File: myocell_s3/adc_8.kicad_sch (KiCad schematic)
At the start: 79 parts, among them U2 ADS1298xPAG

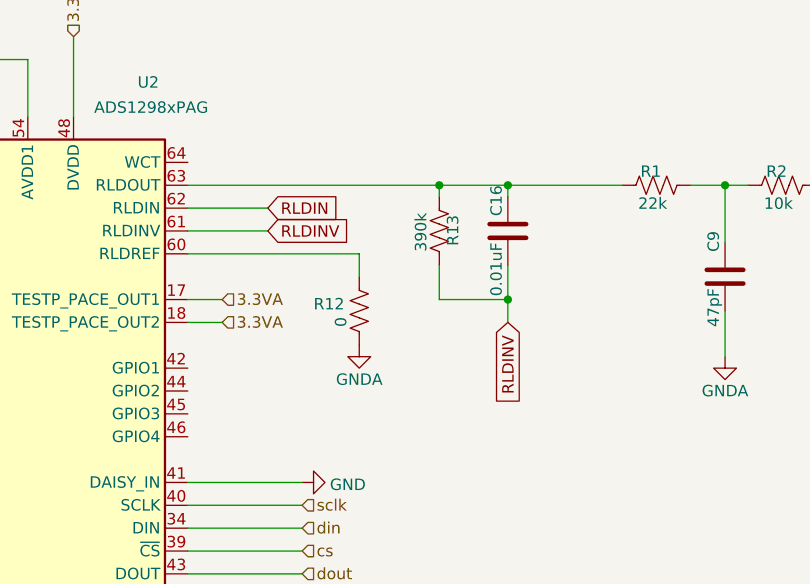
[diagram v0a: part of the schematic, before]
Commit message: schematic and footprints done
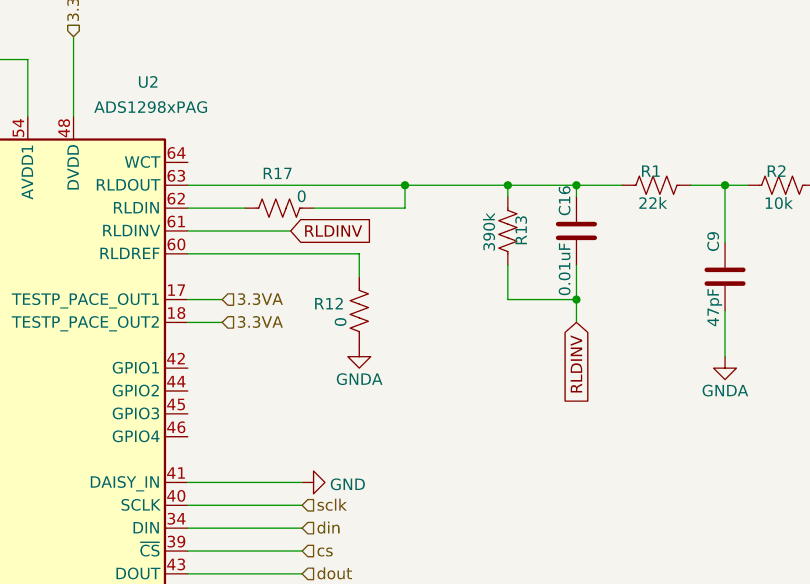
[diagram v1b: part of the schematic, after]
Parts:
- added R17: 0, Resistor_SMD:R_0805_2012Metric_Pad1.20x1.40mm_HandSolder, symbol Device:R_US
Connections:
- net at C16.2, R1.1, R13.1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: now also R17.1
- net RLDIN: no longer names the net of U2.62 (RLDIN)
- net RLDIN: now also R17.2
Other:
- moved on the sheet: C16, R13
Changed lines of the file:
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@@
 	)
 	(junction
-		(at 205.74 53.34)
+		(at 213.36 53.34)
 		(diameter 0)
 		(color 0 0 0 0)
@@
 	)
 	(junction
-		(at 213.36 53.34)
+		(at 220.98 53.34)
 		(diameter 0)
 		(color 0 0 0 0)
 	)
 	(junction
-		(at 213.36 66.04)
+		(at 201.93 53.34)
+		(diameter 0)
+		(color 0 0 0 0)
+	)
+	(junction
+		(at 220.98 66.04)
 		(diameter 0)
 		(color 0 0 0 0)
@@
 	(wire
 		(pts
-			(xy 205.74 66.04) (xy 205.74 62.23)
+			(xy 213.36 66.04) (xy 213.36 62.23)
 		)
 		(stroke
@@
 	(wire
 		(pts
-			(xy 213.36 66.04) (xy 213.36 68.58)
+			(xy 220.98 66.04) (xy 220.98 68.58)
 		)
 		(stroke
@@
 	(wire
 		(pts
-			(xy 213.36 53.34) (xy 226.06 53.34)
+			(xy 220.98 53.34) (xy 226.06 53.34)
 		)
 		(stroke
@@
 	(wire
 		(pts
-			(xy 213.36 62.23) (xy 213.36 66.04)
+			(xy 220.98 62.23) (xy 220.98 66.04)
 		)
 		(stroke
@@
 	(wire
 		(pts
-			(xy 177.8 55.88) (xy 186.69 55.88)
+			(xy 177.8 55.88) (xy 184.15 55.88)
 		)
 		(stroke
@@
 	(wire
 		(pts
+			(xy 201.93 53.34) (xy 213.36 53.34)
+		)
+		(stroke
+			(width 0)
+			(type default)
+		)
+	)
+	(wire
+		(pts
 			(xy 31.75 138.43) (xy 31.75 137.16)
 		)
@@
 	(wire
 		(pts
-			(xy 177.8 53.34) (xy 205.74 53.34)
+			(xy 177.8 53.34) (xy 201.93 53.34)
 		)
 		(stroke
@@
 	(wire
 		(pts
-			(xy 205.74 53.34) (xy 213.36 53.34)
+			(xy 213.36 53.34) (xy 220.98 53.34)
 		)
 		(stroke
@@
 	(wire
 		(pts
-			(xy 177.8 58.42) (xy 186.69 58.42)
+			(xy 177.8 58.42) (xy 189.23 58.42)
 		)
 		(stroke
@@
 	(wire
 		(pts
+			(xy 201.93 55.88) (xy 201.93 53.34)
+		)
+		(stroke
+			(width 0)
+			(type default)
+		)
+	)
+	(wire
+		(pts
 			(xy 59.69 83.82) (xy 59.69 85.09)
 		)
@@
 	(wire
 		(pts
-			(xy 205.74 53.34) (xy 205.74 54.61)
+			(xy 213.36 53.34) (xy 213.36 54.61)
 		)
 		(stroke
@@
 	(wire
 		(pts
-			(xy 213.36 53.34) (xy 213.36 54.61)
+			(xy 220.98 53.34) (xy 220.98 54.61)
 		)
 		(stroke
@@
 	(wire
 		(pts
+			(xy 191.77 55.88) (xy 201.93 55.88)
+		)
+		(stroke
+			(width 0)
+			(type default)
+		)
+	)
+	(wire
+		(pts
 			(xy 270.51 121.92) (xy 264.16 121.92)
 		)
@@
 	(wire
 		(pts
-			(xy 213.36 66.04) (xy 205.74 66.04)
+			(xy 220.98 66.04) (xy 213.36 66.04)
 		)
 		(stroke
@@
 	(global_label "RLDINV"
 		(shape input)
-		(at 213.36 68.58 270)
+		(at 220.98 68.58 270)
 		(fields_autoplaced yes)
 		(effects
@@
 		)
 		(property "Intersheetrefs" "${INTERSHEET_REFS}"
-			(at 213.36 78.1572 90)
+			(at 220.98 78.1572 90)
 			(effects
 				(font
@@
 	(global_label "RLDINV"
 		(shape input)
-		(at 186.69 58.42 0)
-		(fields_autoplaced yes)
-		(effects
-			(font
-				(size 1.27 1.27)
-			)
-			(justify left)
-		)
-		(property "Intersheetrefs" "${INTERSHEET_REFS}"
-			(at 196.2672 58.42 0)
-			(effects
-				(font
-					(size 1.27 1.27)
-				)
-				(justify left)
-				(hide yes)
-			)
-		)
-	)
-	(global_label "RLDIN"
-		(shape input)
-		(at 186.69 55.88 0)
+		(at 189.23 58.42 0)
 		(fields_autoplaced yes)
 		(effects
@@
 		)
 		(property "Intersheetrefs" "${INTERSHEET_REFS}"
-			(at 195.1786 55.88 0)
+			(at 198.8072 58.42 0)
 			(effects
 				(font
@@
 	(symbol
 		(lib_id "Device:C")
-		(at 213.36 58.42 180)
+		(at 220.98 58.42 180)
 		(unit 1)
 		(exclude_from_sim no)
@@
 		(dnp no)
 		(property "Reference" "C16"
-			(at 212.09 53.34 90)
+			(at 219.71 53.34 90)
 			(effects
 				(font
@@
 		)
 		(property "Value" "0.01uF"
-			(at 212.09 59.69 90)
+			(at 219.71 59.69 90)
 			(effects
 				(font
@@
 		)
 		(property "Footprint" "Capacitor_SMD:C_0805_2012Metric_Pad1.18x1.45mm_HandSolder"
-			(at 212.3948 54.61 0)
+			(at 220.0148 54.61 0)
 			(effects
 				(font
@@
 		)
 		(property "Datasheet" "~"
-			(at 213.36 58.42 0)
+			(at 220.98 58.42 0)
 			(effects
 				(font
@@
 		)
 		(property "Description" "Unpolarized capacitor"
-			(at 213.36 58.42 0)
+			(at 220.98 58.42 0)
 			(effects
 				(font
@@
 	(symbol
 		(lib_id "Device:R_US")
-		(at 205.74 58.42 0)
+		(at 213.36 58.42 0)
 		(unit 1)
 		(exclude_from_sim no)
@@
 		(dnp no)
 		(property "Reference" "R13"
-			(at 207.264 56.642 90)
+			(at 214.884 56.642 90)
 			(effects
 				(font
@@
 		)
 		(property "Value" "390k"
-			(at 203.708 56.388 90)
+			(at 211.328 56.388 90)
 			(effects
 				(font
@@
 		)
 		(property "Footprint" "Resistor_SMD:R_0805_2012Metric_Pad1.20x1.40mm_HandSolder"
-			(at 206.756 58.674 90)
+			(at 214.376 58.674 90)
 			(effects
 				(font
@@
 		)
 		(property "Datasheet" "~"
-			(at 205.74 58.42 0)
+			(at 213.36 58.42 0)
 			(effects
 				(font
@@
 		)
 		(property "Description" "Resistor, US symbol"
-			(at 205.74 58.42 0)
+			(at 213.36 58.42 0)
 			(effects
 				(font
@@
 					(unit 1)
 				)
+			)
+		)
+	)
+	(symbol
+		(lib_id "Device:R_US")
+		(at 187.96 55.88 270)
+		(unit 1)
+		(exclude_from_sim no)
+		(in_bom yes)
+		(on_board yes)
+		(dnp no)
+		(property "Reference" "R17"
+			(at 189.484 52.07 90)
+			(effects
+				(font
+					(size 1.27 1.27)
+				)
+				(justify right)
+			)
+		)
+		(property "Value" "0"
+			(at 191.008 54.61 90)
+			(effects
+				(font
+					(size 1.27 1.27)
+				)
+				(justify right)
+			)
+		)
+		(property "Footprint" "Resistor_SMD:R_0805_2012Metric_Pad1.20x1.40mm_HandSolder"
+			(at 187.706 56.896 90)
+			(effects
+				(font
+					(size 1.27 1.27)
+				)
+				(hide yes)
+			)
+		)
+		(property "Datasheet" "~"
+			(at 187.96 55.88 0)
+			(effects
+				(font
+					(size 1.27 1.27)
+				)
+				(hide yes)
+			)
+		)
+		(property "Description" "Resistor, US symbol"
+			(at 187.96 55.88 0)
+			(effects
+				(font
+					(size 1.27 1.27)
+				)
+				(hide yes)
+			)
+		)
+		(pin "1"
+		)
+		(pin "2"
+		)
+		(instances
+			(project "myocell_s3"
+				(path "/871ff10b-bde5-471c-b91a-de58aa271388/c595076a-24ce-4f55-8e02-687765014fdd"
+					(reference "R17")
+					(unit 1)
+				)

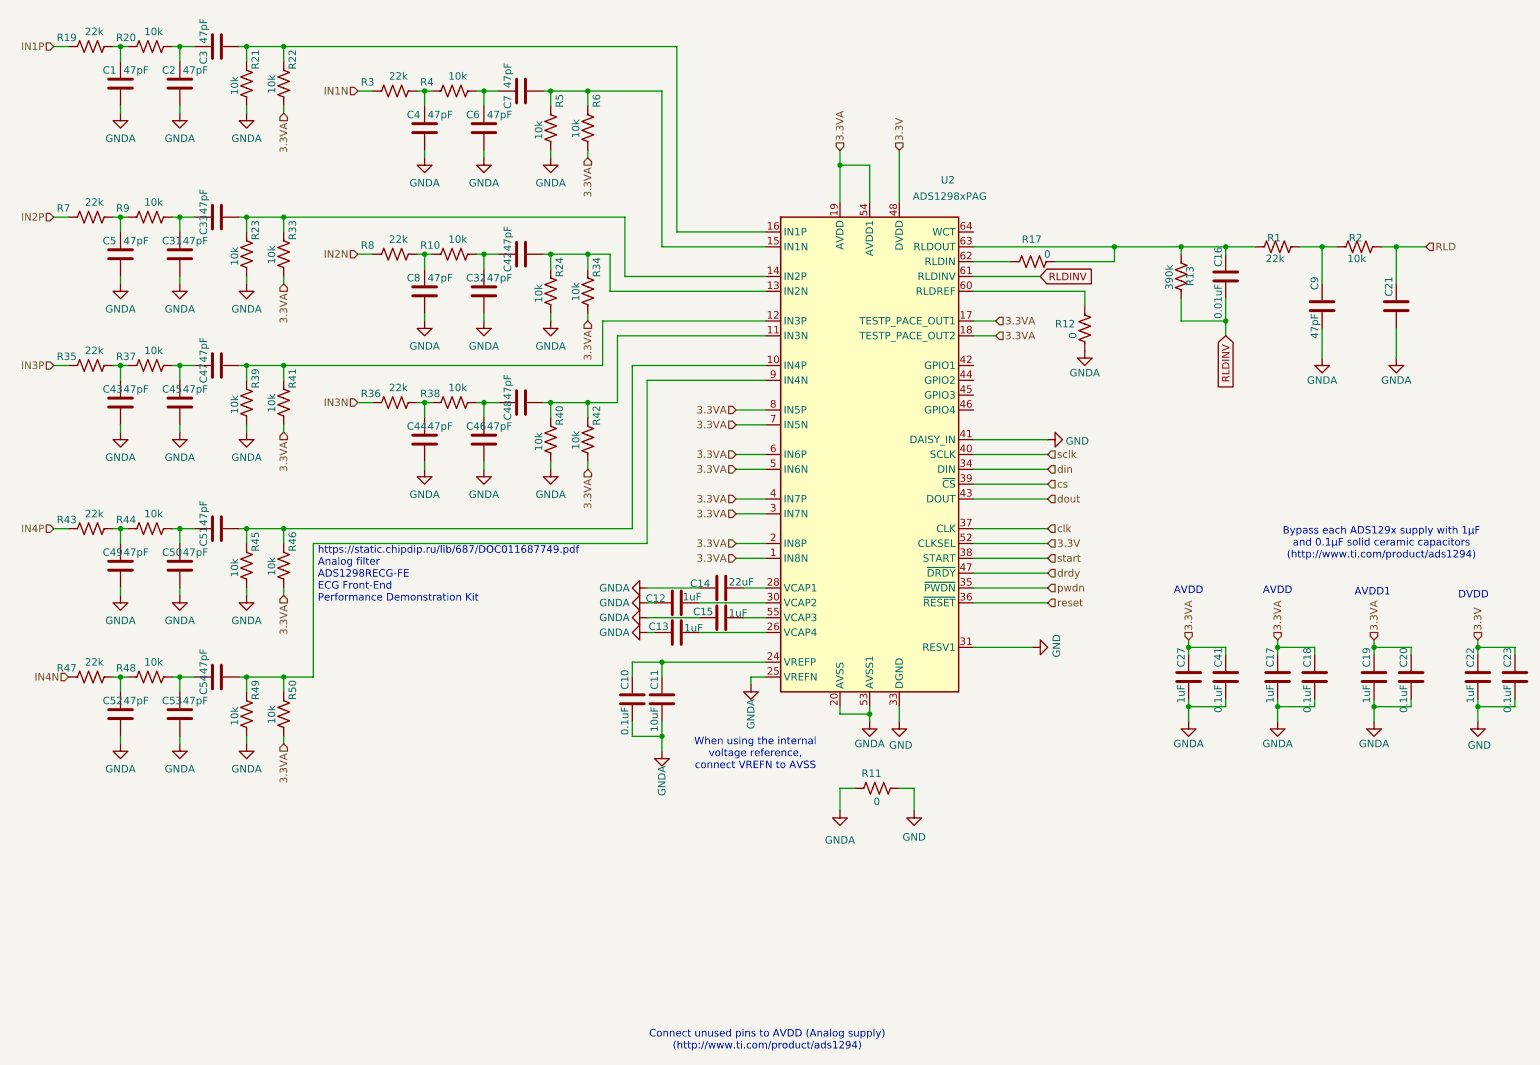
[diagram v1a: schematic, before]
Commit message: working on parts placement
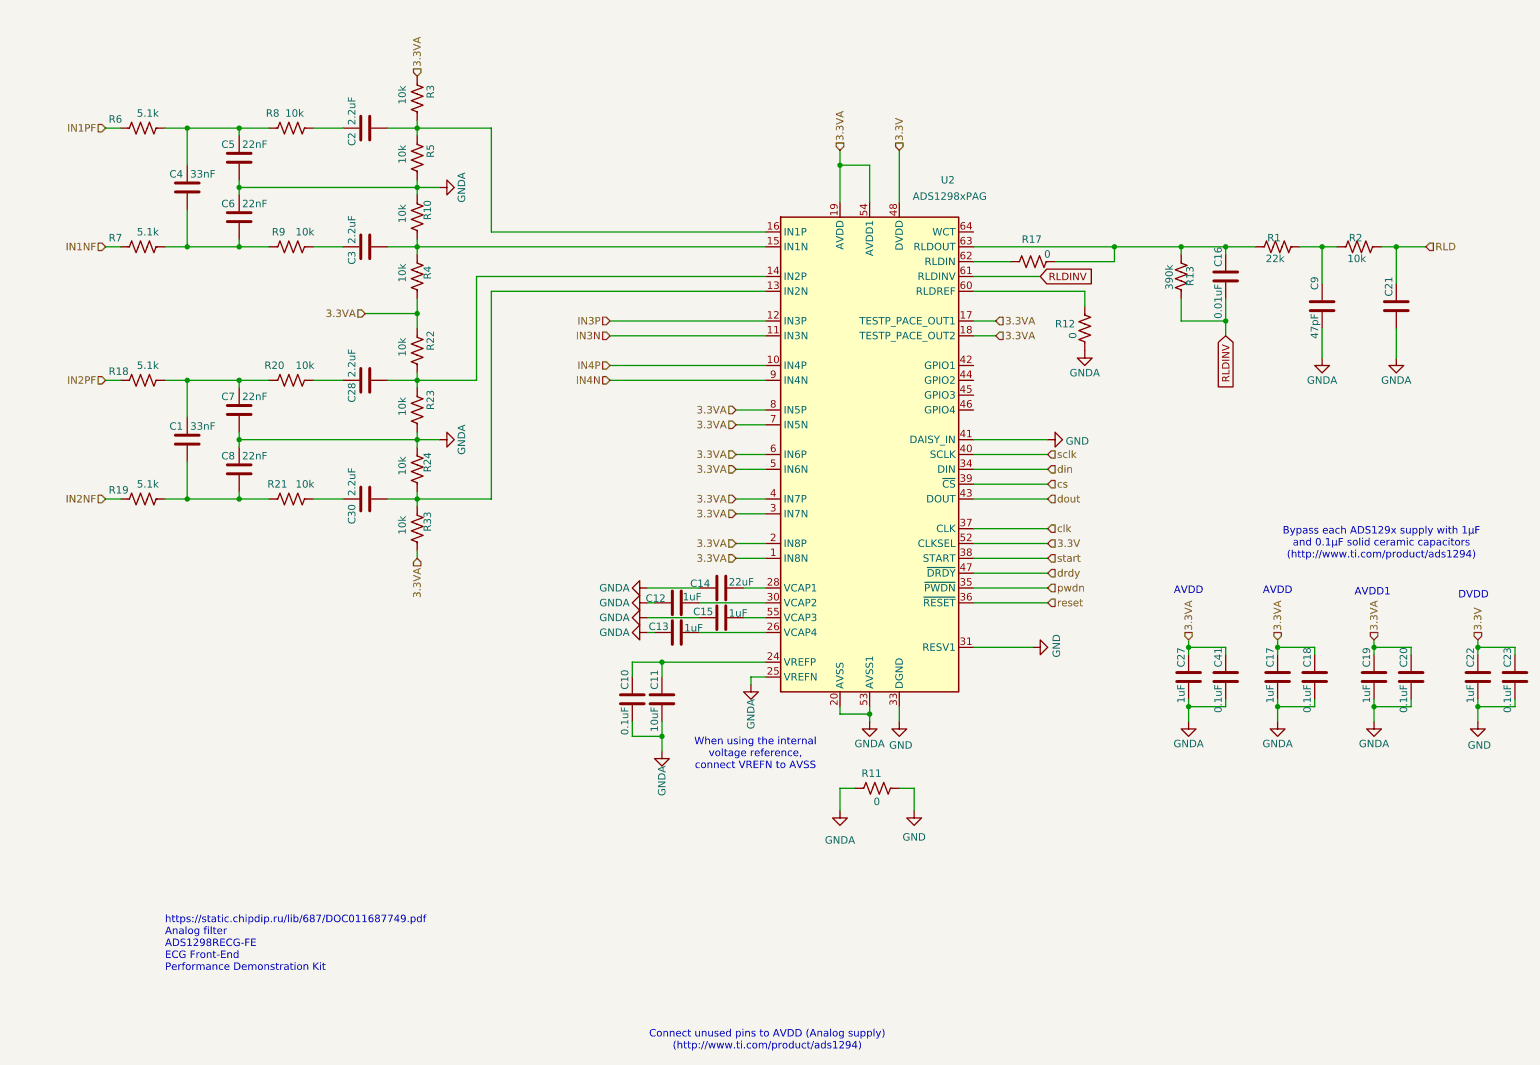
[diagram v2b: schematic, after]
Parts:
- removed C31, C32, C33, C42, C43, C44, C45, C46, C47, C48, C49, C50, C51, C52, C53, C54: 47pF, Capacitor_SMD:C_0805_2012Metric_Pad1.18x1.45mm_HandSolder, symbol Device:C
- removed R34, R37, R38, R39, R40, R41, R42, R44, R45, R46, R48, R49, R50: 10k, Resistor_SMD:R_0805_2012Metric_Pad1.20x1.40mm_HandSolder, symbol Device:R_US
- removed R35, R36, R43, R47: 22k, Resistor_SMD:R_0805_2012Metric_Pad1.20x1.40mm_HandSolder, symbol Device:R_US
- added C28, C30: 2.2uF, Capacitor_SMD:C_0805_2012Metric_Pad1.18x1.45mm_HandSolder, symbol Device:C
- added R18: 5.1k, Resistor_SMD:R_0805_2012Metric_Pad1.20x1.40mm_HandSolder, symbol Device:R_US
- C1, C4: value 47pF -> 33nF
- C2, C3: value 47pF -> 2.2uF
- C5, C6, C7, C8: value 47pF -> 22nF
- R19, R7: value 22k -> 5.1k
- R3, R8: value 22k -> 10k
- R6: value 10k -> 5.1k
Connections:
- net 3.3VA: now also R3.2, R33.1, R4.1; no longer R33.2, R6.2
- net GNDA: now also C6.1, C7.2, C8.1, R10.2, R23.1, R5.1; no longer C1.2, C2.2, C4.2, C6.2, C8.2, R21.2, R23.2, R5.2
- net IN3N: now also U2.11 (IN3N)
- net IN3P: now also U2.12 (IN3P)
- net IN4N: now also U2.9 (IN4N)
- net IN4P: now also U2.10 (IN4P)
- net at R9.2: now also C3.1
- net at R24.1, U2.13 (IN2N): now also R33.2, C30.2
- net at C1.1, R20.1: now also C7.1, R18.2; no longer R19.2
- net at R7.2, R9.1: now also C4.2, C6.2; no longer C5.1
- net IN1N: no longer names the net of R3.1
- net IN1N: now also C2.2, R5.2, U2.16 (IN1P)
- net IN1P renamed IN2NF
- net IN2N: no longer names the net of R8.1
- net IN2N: now also C4.1, C5.1, R6.2
- net IN2P renamed IN1NF
- new net: C3.2, R10.1, R4.2, U2.15 (IN1N)
- new net: C28.2, R22.1, R23.2, U2.14 (IN2P)
- new net: C2.1, R8.2
- new net: C28.1, R20.2
- new net: C1.2, C8.2, R19.2, R21.1
- new net: C30.1, R21.2
- new net IN1PF: R6.1
- new net IN2PF: R18.1
